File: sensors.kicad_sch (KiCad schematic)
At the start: 13 parts, among them U11 LPS22DF, U4 LSM6DSO32TR, U7 LSM6DSO32TR, U8 LIS2MDL

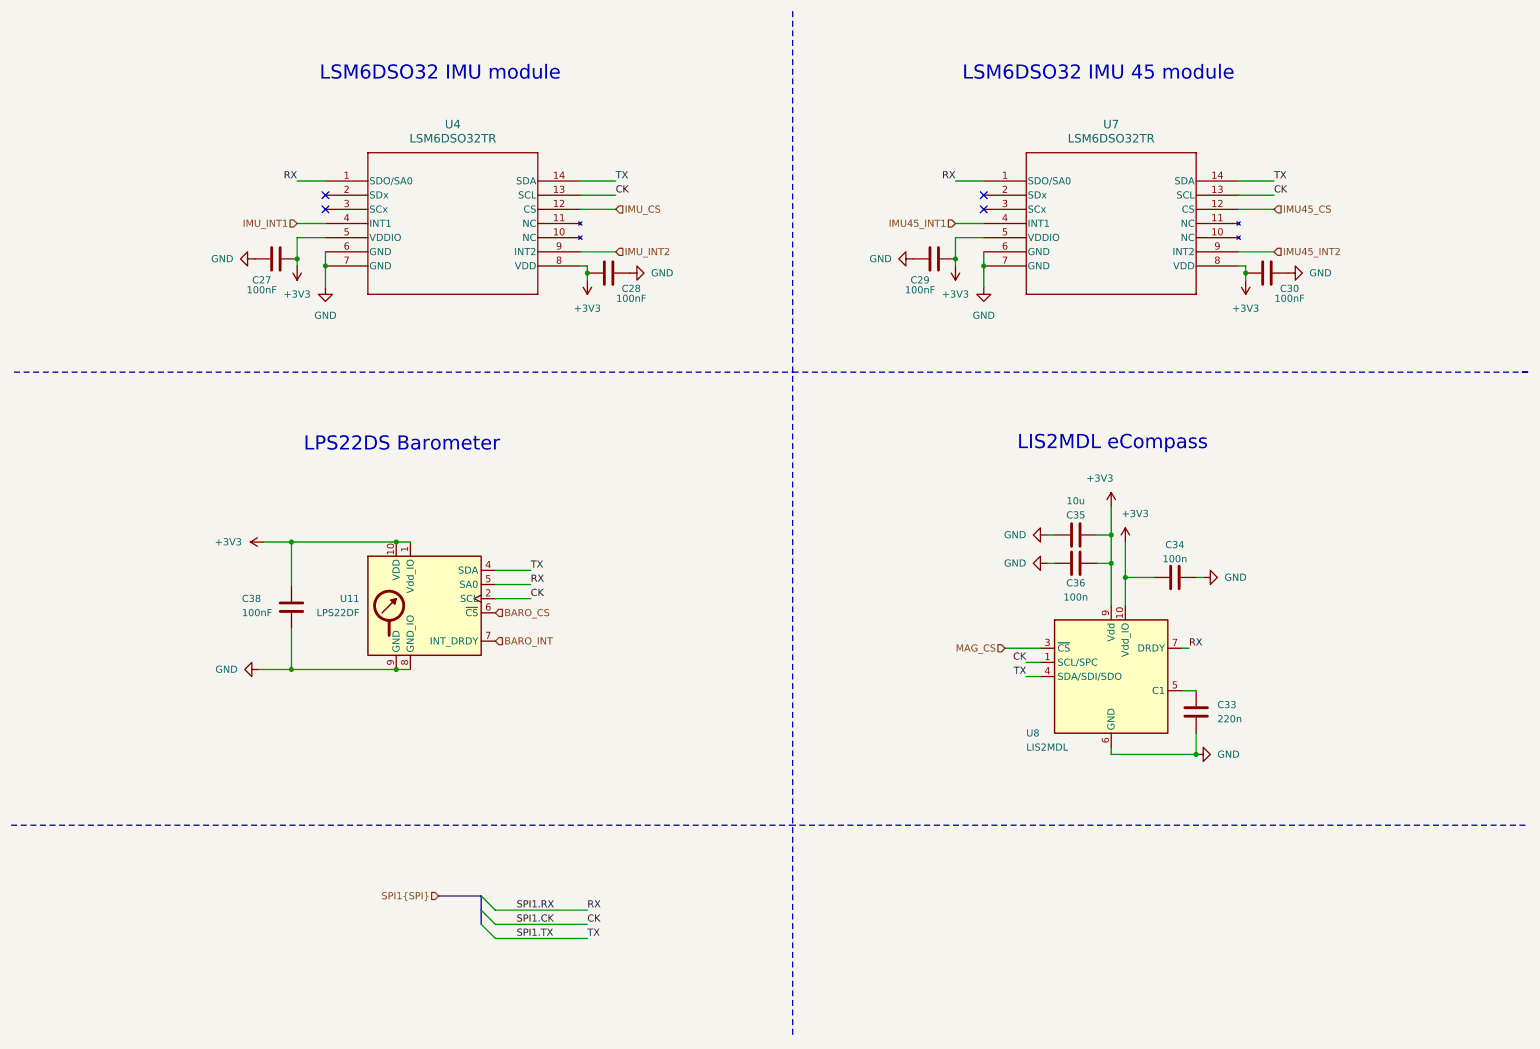
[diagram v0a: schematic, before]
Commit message: ROBE
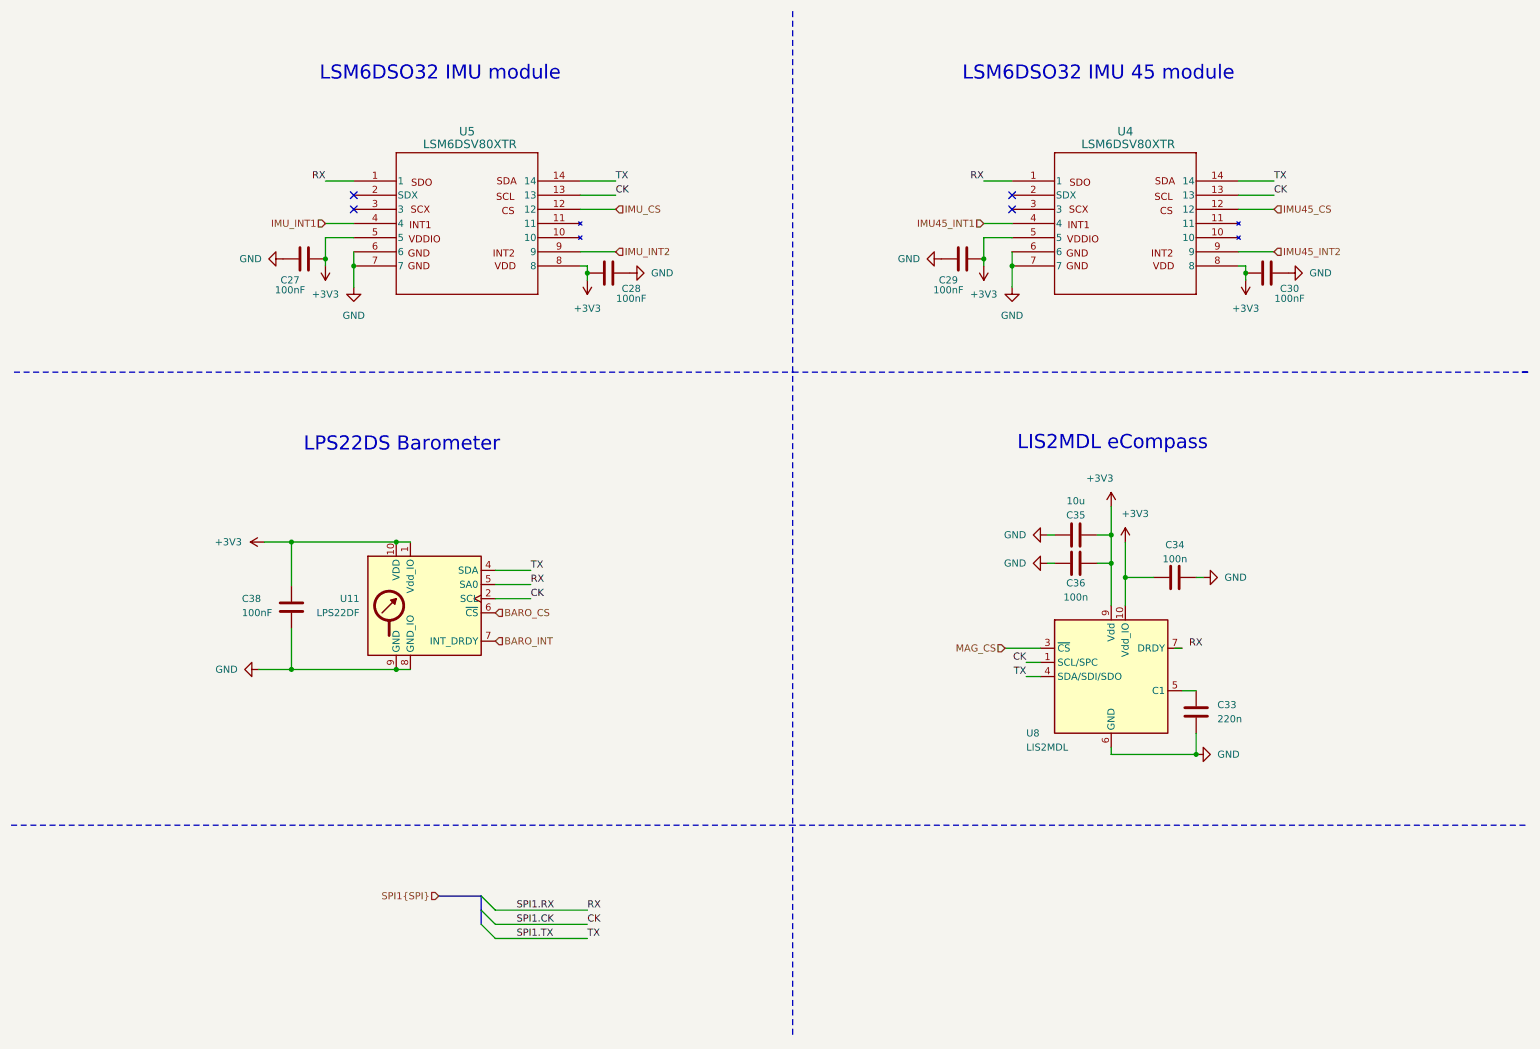
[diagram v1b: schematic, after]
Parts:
- removed U4, U7: LSM6DSO32TR, LSM6DSO32TR:LGA-14L_2P5X3X0P83_STM-M, symbol 2024-10-18_09-38-35:LSM6DSO32TR
- added U4, U5: LSM6DSV80XTR, lsm6dsv80x:QFN_LSM6DSV80XTR_STM, symbol lsm6dsv80x:LSM6DSV80XTR
- U11: footprint Package_LGA:ST_HLGA-10_2x2mm_P0.5mm_LayoutBorder3x2y -> LPS22DF:ST_HLGA-10_2x2mm_P0.5mm_LayoutBorder3x2y
- U8: footprint Package_LGA:LGA-12_2x2mm_P0.5mm -> LIS2MDL:LGA-12_2x2mm_P0.5mm
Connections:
- net +3V3: now also U4.5, U4.8, U5.5, U5.8
- net CK: now also U4.13, U5.13
- net GND: now also U4.6, U4.7, U5.6, U5.7
- net IMU45_CS: now also U4.12
- net IMU45_INT1: now also U4.4
- net IMU45_INT2: now also U4.9
- net IMU_CS: now also U5.12
- net IMU_INT1: now also U5.4
- net IMU_INT2: now also U5.9
- net RX: now also U4.1, U5.1; no longer U8.7 (DRDY)
- net SPI1.TX: now also U4.14, U5.14
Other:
- moved on the sheet: C27, C29
